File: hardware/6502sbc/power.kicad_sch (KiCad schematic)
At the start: 21 parts, among them J20 +5VDC, J21 Clock input, U21 LD1117STR, U22 LD1117S33TR_SOT223, U23 74AHC2G00, U5 SN74LS07

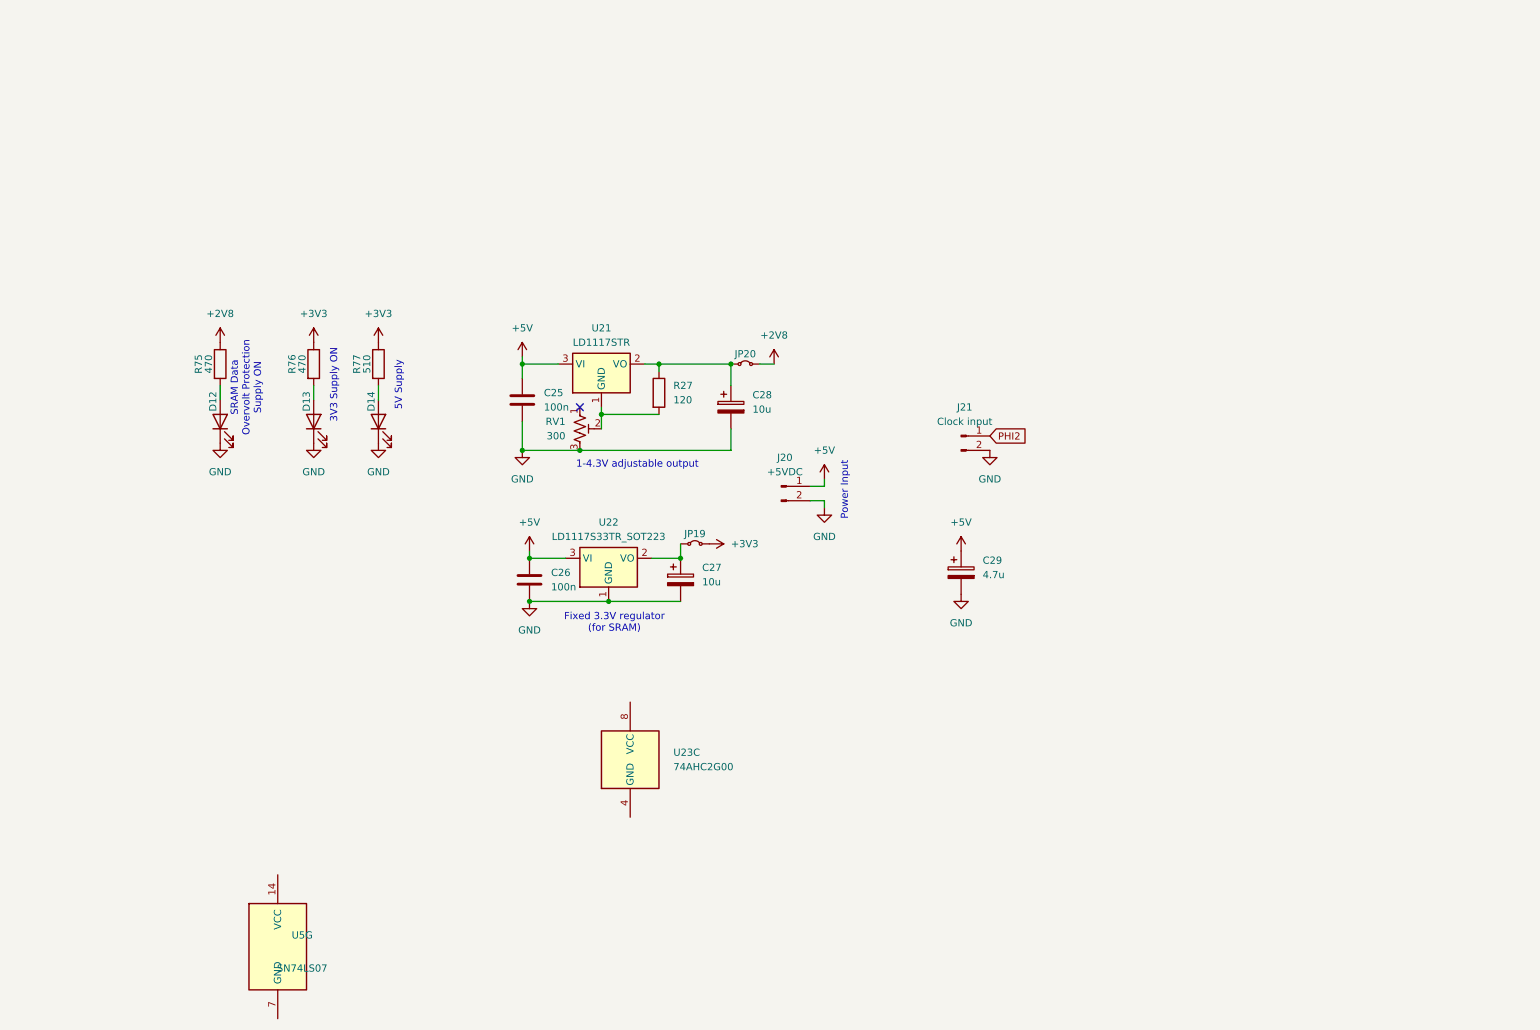
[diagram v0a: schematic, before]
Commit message: Schematic is nearly done
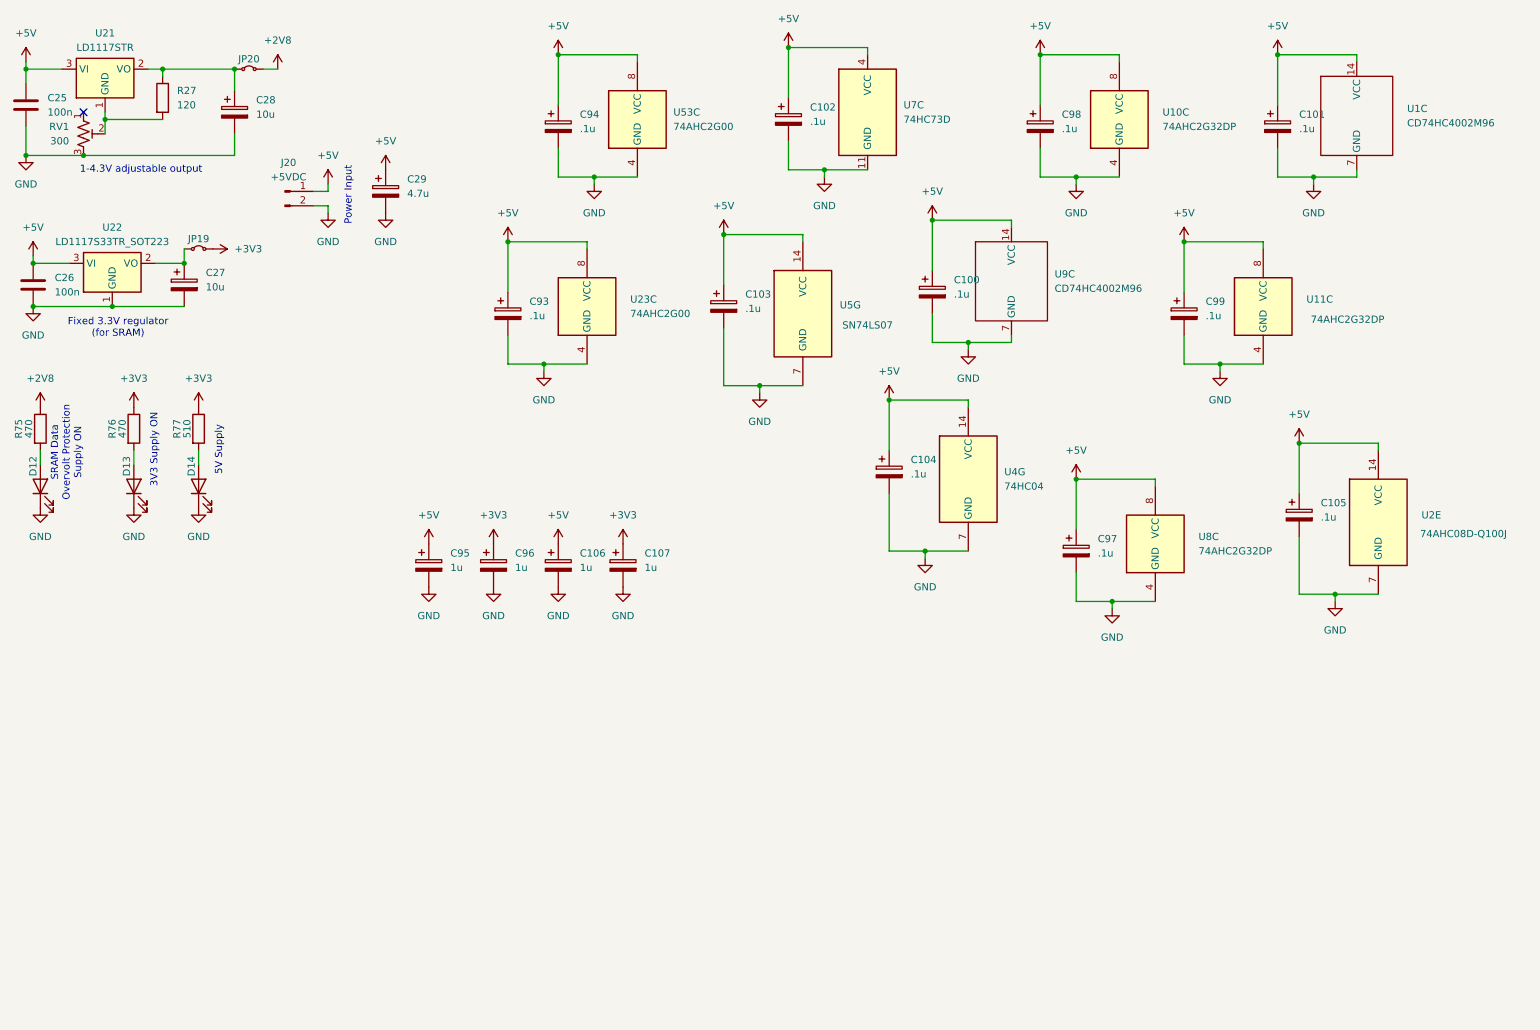
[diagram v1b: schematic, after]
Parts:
- removed J21: Clock input, symbol Connector:Conn_01x02_Pin
- added C100, C101, C102, C103, C104, C105, C93, C94, C97, C98, C99: .1u, symbol Device:C_Polarized
- added C106, C107, C95, C96: 1u, symbol Device:C_Polarized
- added U1, U9: CD74HC4002M96, Package_SO:SOIC-14_3.9x8.7mm_P1.27mm, symbol custom:_1
- added U10, U11, U8: 74AHC2G32DP, Package_SO:TSSOP-8_3x3mm_P0.65mm, symbol 74xGxx:74LVC2G32
- added U2: 74AHC08D-Q100J, Package_SO:SOIC-14_3.9x8.7mm_P1.27mm, symbol 74xx:74LS08
- added U4: 74HC04, Package_SO:SOIC-14_3.9x8.7mm_P1.27mm, symbol 74xx:74HC04
- added U53: 74AHC2G00, symbol 74xGxx:74AHC2G00
- added U7: 74HC73D, Package_SO:SOIC-14_3.9x8.7mm_P1.27mm, symbol 74xx:74LS73
- U5: footprint (none) -> Package_SO:SOIC-14_3.9x8.7mm_P1.27mm; t_pd (ns) (none) -> 30
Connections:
- net +3V3: now also C107.1, C96.1
- net +5V: now also U23.8 (VCC), U5.14 (VCC), C100.1, C101.1, C102.1, C103.1, C104.1, C105.1, C106.1, C93.1, C94.1, C95.1, C97.1, C98.1, C99.1, U1.14 (VCC), U10.8 (VCC), U11.8 (VCC), U2.14 (VCC), U4.14 (VCC), U53.8 (VCC), U7.4 (VCC), U8.8 (VCC), U9.14 (VCC)
- net GND: now also U23.4 (GND), U5.7 (GND), C100.2, C101.2, C102.2, C103.2, C104.2, C105.2, C106.2, C107.2, C93.2, C94.2, C95.2, C96.2, C97.2, C98.2, C99.2, U1.7 (GND), U10.4 (GND), U11.4 (GND), U2.7 (GND), U4.7 (GND), U53.4 (GND), U7.11 (GND), U8.4 (GND), U9.7 (GND)
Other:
- moved on the sheet: C25, C26, C27, C28, C29, D12, D13, D14, J20, JP19, JP20, R27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
